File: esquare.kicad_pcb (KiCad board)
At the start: 2 copper layers, 21.3 x 27.8 mm, 11 parts

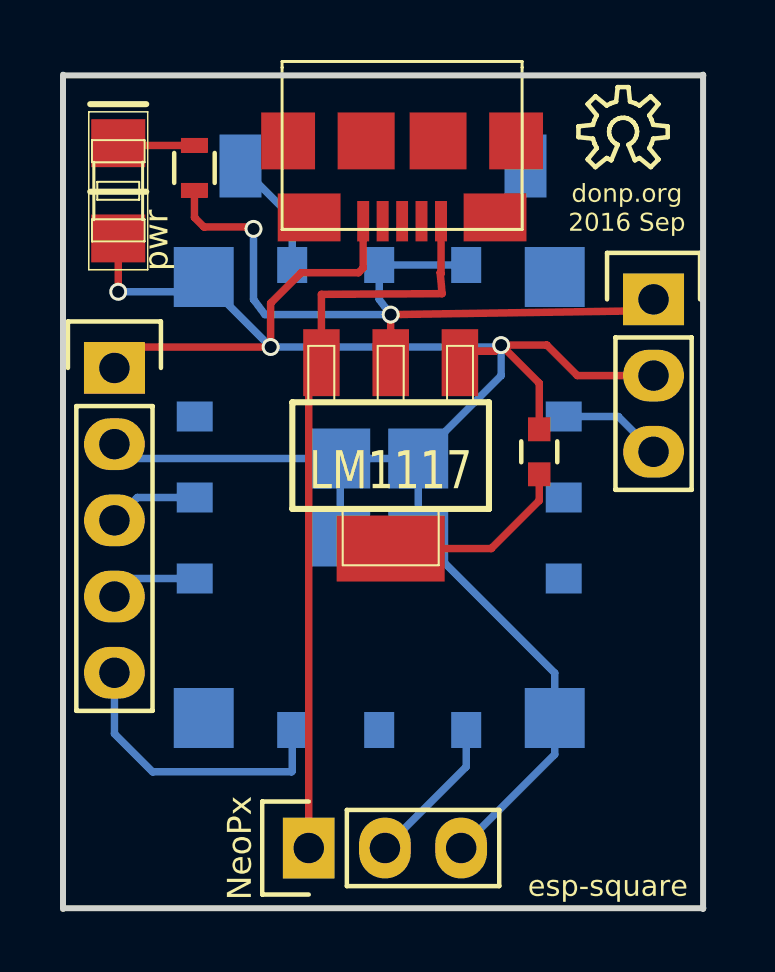
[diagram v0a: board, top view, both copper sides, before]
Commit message: square rev b
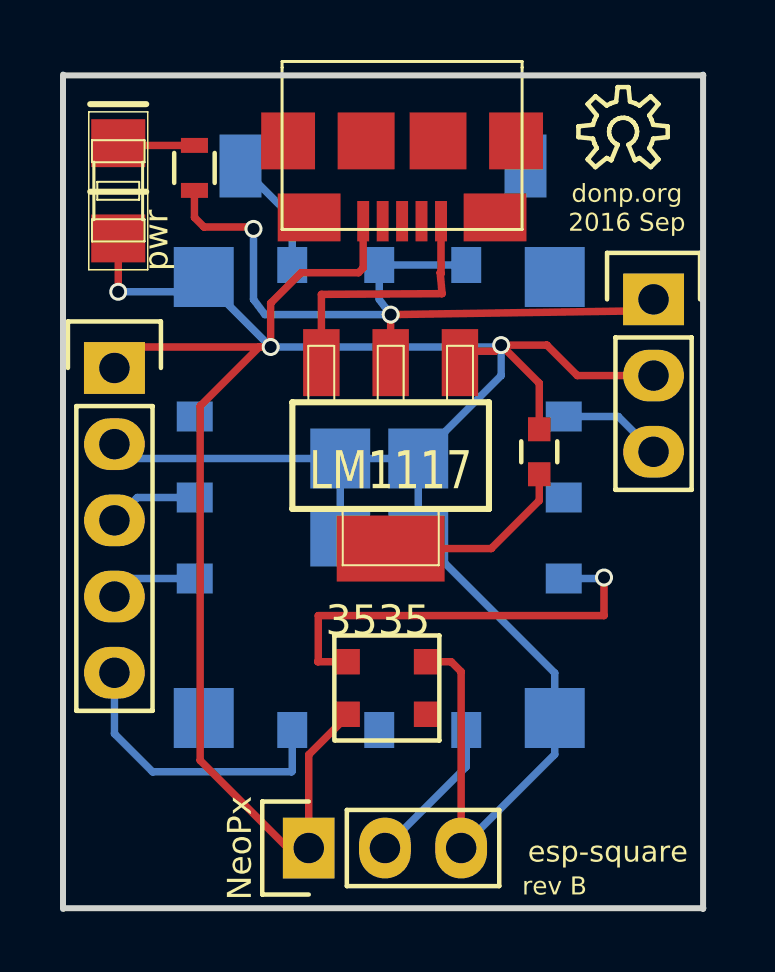
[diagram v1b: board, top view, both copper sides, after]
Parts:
- added 3535: 3535, ws2812:3535, F.Cu at (142.7, 58.4)
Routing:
- net (no net): track 162.3 -> 194.0 mm, vias 5 -> 6
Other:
- board text added: "rev B"
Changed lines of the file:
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@@
     (area 123.678215 35.86461 161.627286 73.743285)
     (thickness 1.6)
-    (drawings 6)
-    (tracks 80)
+    (drawings 7)
+    (tracks 99)
     (zones 0)
-    (modules 11)
+    (modules 12)
     (nets 1)
   )
@@
     )
   )
-  (gr_text esp-square (at 150.114 65.024) (layer F.SilkS)
+  (module ws2812:3535 (layer F.Cu)
+    (at 142.748 58.42 180)
+    (fp_text reference 3535 (at 0.3 2.25 180) (layer F.SilkS)
+      (effects (font (size 1 1) (thickness 0.15)))
+    )
+    (fp_text value 3535 (at 0.05 -2.2 180) (layer F.Fab)
+      (effects (font (size 1 1) (thickness 0.15)))
+    )
+    (fp_line (start 1.75 1.75) (end -1.75 1.75) (layer F.SilkS) (width 0.15))
+    (fp_line (start -1.75 1.75) (end -1.75 -1.75) (layer F.SilkS) (width 0.15))
+    (fp_line (start 1.75 -1.75) (end 1.75 1.75) (layer F.SilkS) (width 0.15))
+    (fp_line (start -1.75 -1.75) (end 1.7 -1.75) (layer F.SilkS) (width 0.15))
+    (pad IN smd rect (at 1.325 0.875 180) (size 0.85 0.85) (layers F.Cu F.Paste F.Mask))
+    (pad VDD smd rect (at 1.325 -0.875 180) (size 0.85 0.85) (layers F.Cu F.Paste F.Mask))
+    (pad VSS smd rect (at -1.325 0.875 180) (size 0.85 0.85) (layers F.Cu F.Paste F.Mask))
+    (pad OUT smd rect (at -1.325 -0.875 180) (size 0.85 0.85) (layers F.Cu F.Paste F.Mask))
+  )
+  (gr_text "rev B" (at 148.336 65.024) (layer F.SilkS)
+    (effects (font (size 0.6 0.6) (thickness 0.1)))
+  )
+  (gr_text esp-square (at 150.114 63.881) (layer F.SilkS)
     (effects (font (size 0.7 0.7) (thickness 0.1)))
   )
@@
     (effects (font (size 0.6 0.6) (thickness 0.1)))
   )
-  (segment (start 140.56614 47.5742) (end 140.56614 48.15586) (width 0.25) (layer F.Cu) (net 0) (status C00000))
-  (segment (start 140.56614 48.15586) (end 140.1445 48.5775) (width 0.25) (layer F.Cu) (net 0) (status C00000))
-  (segment (start 140.1445 48.5775) (end 140.1445 63.754) (width 0.25) (layer F.Cu) (net 0) (status C00000))
-  (segment (start 145.394 59.82) (end 145.394 61.0445) (width 0.25) (layer B.Cu) (net 0) (status 400000))
-  (segment (start 145.394 61.0445) (end 142.6845 63.754) (width 0.25) (layer B.Cu) (net 0) (status 800000))
-  (segment (start 148.344 59.42) (end 148.344 60.6345) (width 0.25) (layer B.Cu) (net 0) (status 400000))
-  (segment (start 148.344 60.6345) (end 145.2245 63.754) (width 0.25) (layer B.Cu) (net 0) (status 800000))
+  (segment (start 141.423 57.545) (end 140.448 57.545) (width 0.25) (layer F.Cu) (net 0))
+  (segment (start 149.954 54.77) (end 148.644 54.77) (width 0.25) (layer B.Cu) (net 0))
+  (segment (start 149.987 54.737) (end 149.954 54.77) (width 0.25) (layer B.Cu) (net 0))
+  (via (at 149.987 54.737) (size 0.6) (drill 0.4) (layers F.Cu B.Cu) (net 0))
+  (segment (start 149.987 56.007) (end 149.987 54.737) (width 0.25) (layer F.Cu) (net 0))
+  (segment (start 140.462 56.007) (end 149.987 56.007) (width 0.25) (layer F.Cu) (net 0))
+  (segment (start 140.462 57.531) (end 140.462 56.007) (width 0.25) (layer F.Cu) (net 0))
+  (segment (start 140.448 57.545) (end 140.462 57.531) (width 0.25) (layer F.Cu) (net 0))
+  (segment (start 144.073 57.545) (end 144.893 57.545) (width 0.25) (layer F.Cu) (net 0))
+  (segment (start 145.2245 57.8765) (end 145.2245 63.754) (width 0.25) (layer F.Cu) (net 0))
+  (segment (start 144.893 57.545) (end 145.2245 57.8765) (width 0.25) (layer F.Cu) (net 0))
+  (segment (start 144.073 59.295) (end 144.073 59.508) (width 0.25) (layer F.Cu) (net 0))
+  (segment (start 141.423 59.295) (end 141.423 59.364) (width 0.25) (layer F.Cu) (net 0))
+  (segment (start 141.423 59.364) (end 140.1445 60.6425) (width 0.25) (layer F.Cu) (net 0))
+  (segment (start 140.1445 60.6425) (end 140.1445 63.754) (width 0.25) (layer F.Cu) (net 0))
+  (segment (start 138.8745 47.0535) (end 138.4935 47.0535) (width 0.25) (layer F.Cu) (net 0))
+  (segment (start 136.525 60.833) (end 139.446 63.754) (width 0.25) (layer F.Cu) (net 0))
+  (segment (start 136.525 49.022) (end 136.525 60.833) (width 0.25) (layer F.Cu) (net 0))
+  (segment (start 138.4935 47.0535) (end 136.525 49.022) (width 0.25) (layer F.Cu) (net 0))
+  (segment (start 139.446 63.754) (end 140.1445 63.754) (width 0.25) (layer F.Cu) (net 0))
+  (segment (start 140.56614 47.5742) (end 140.56614 48.15586) (width 0.25) (layer F.Cu) (net 0))
+  (segment (start 140.56614 48.15586) (end 140.1445 48.5775) (width 0.25) (layer F.Cu) (net 0))
+  (segment (start 145.394 59.82) (end 145.394 61.0445) (width 0.25) (layer B.Cu) (net 0))
+  (segment (start 145.394 61.0445) (end 142.6845 63.754) (width 0.25) (layer B.Cu) (net 0))
+  (segment (start 148.344 59.42) (end 148.344 60.6345) (width 0.25) (layer B.Cu) (net 0))
+  (segment (start 148.344 60.6345) (end 145.2245 63.754) (width 0.25) (layer B.Cu) (net 0))
   (segment (start 148.644 49.37) (end 150.462 49.37) (width 0.25) (layer B.Cu) (net 0))
   (segment (start 150.462 49.37) (end 151.638 50.546) (width 0.25) (layer B.Cu) (net 0))
@@
   (segment (start 138.303 45.466) (end 138.303 43.1165) (width 0.25) (layer B.Cu) (net 0))
   (segment (start 138.684 45.974) (end 138.303 45.466) (width 0.25) (layer B.Cu) (net 0))
-  (segment (start 142.875 47.5742) (end 142.875 45.974) (width 0.25) (layer F.Cu) (net 0) (status 400010))
+  (segment (start 142.875 47.5742) (end 142.875 45.974) (width 0.25) (layer F.Cu) (net 0) (status 10))
   (segment (start 142.494 45.466) (end 142.494 44.32) (width 0.25) (layer B.Cu) (net 0) (status 20))
   (segment (start 142.875 45.974) (end 142.494 45.466) (width 0.25) (layer B.Cu) (net 0))
